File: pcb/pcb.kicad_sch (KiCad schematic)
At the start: 71 parts, among them J1 WH, J2 RGB, J3 220, Q1 AO3400A, Q2 AO3400A, Q3 AO3400A, Q4 AO3400A, Q5 AOD452, Q6 DTD114E, Q7 AO3400A, SW1 mode, SW2 bright, T1 ., U1 ATtiny13A-SS, U2 TNY268G, U3 PC817, U4 TL431DBZ, U5 AZ1117-5.0

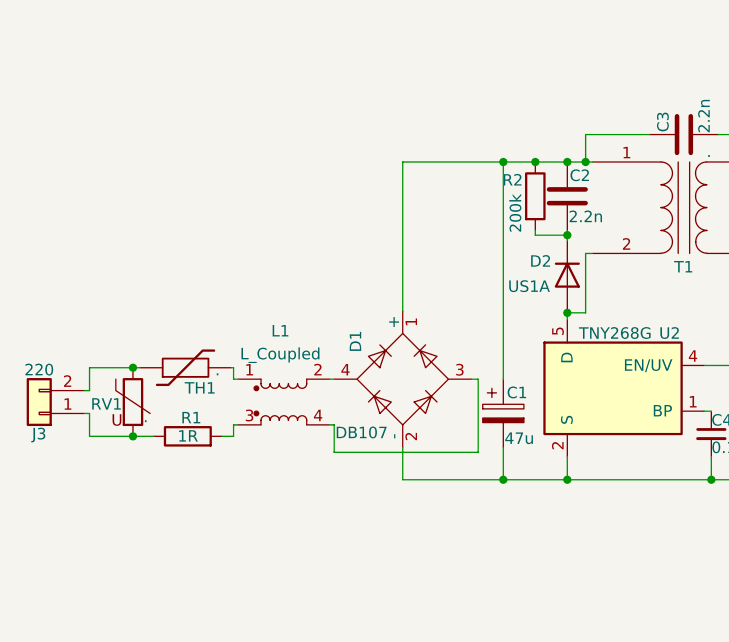
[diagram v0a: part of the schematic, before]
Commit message: -0.5 cm
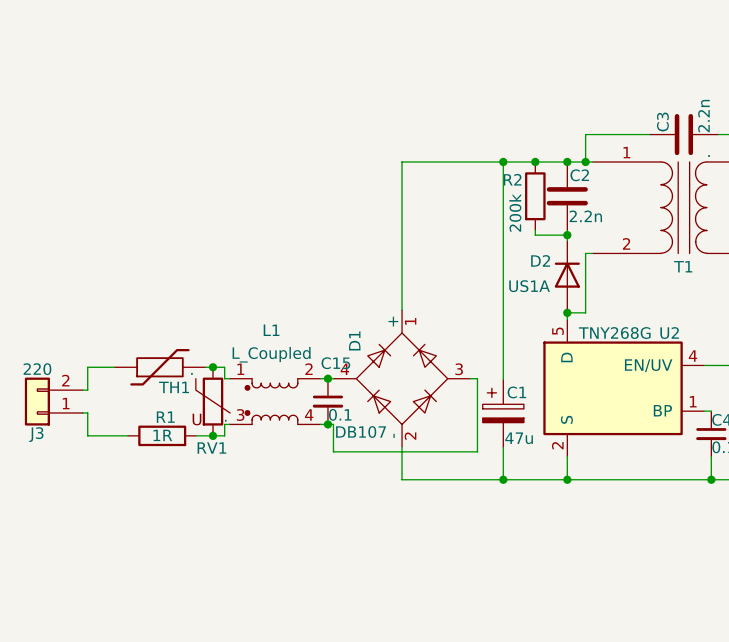
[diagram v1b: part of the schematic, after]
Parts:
- added C15: 0.1, Capacitor_THT:C_Rect_L13.0mm_W6.0mm_P10.00mm_FKS3_FKP3_MKS4, symbol Device:C_Small
- C1: footprint Capacitor_THT:CP_Radial_D13.0mm_P7.50mm -> Capacitor_THT:CP_Radial_D10.0mm_P7.50mm
- L1: footprint Inductor_THT:Choke_Schaffner_RN212-04-12.5x18.0mm -> local:Input_coil
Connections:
- net at J3.2 (Pin_2), TH1.1: no longer RV1.1
- net at J3.1 (Pin_1), R1.1: no longer RV1.2
- net at D1.3, L1.4: now also C15.2
- net at D1.4, L1.2: now also C15.1
- net at L1.1, TH1.2: now also RV1.1
- net at L1.3, R1.2: now also RV1.2
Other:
- moved on the sheet: L1, R1, RV1, TH1
